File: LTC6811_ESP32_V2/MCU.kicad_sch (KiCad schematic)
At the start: 17 parts, among them J18 B2P-VH-B, J8 JTAG /NC, U8 ESP32-DevKitC V4, U9 LTC6820

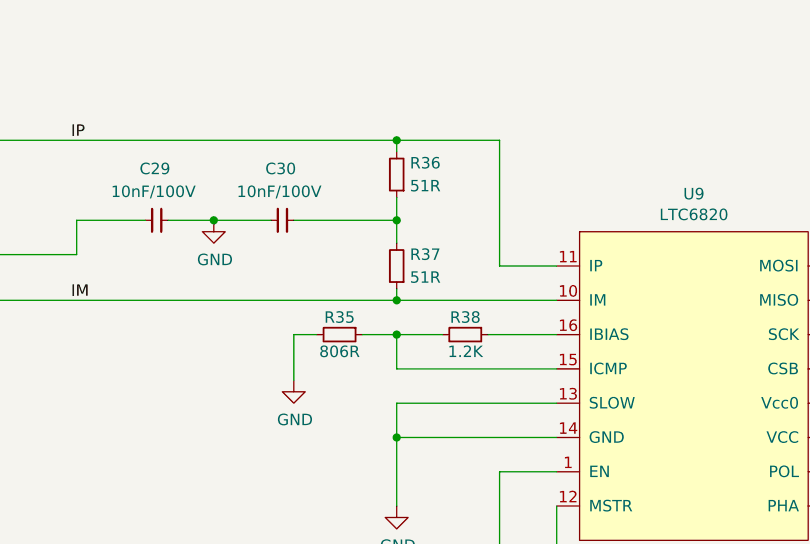
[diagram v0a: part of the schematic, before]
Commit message: Add files via upload
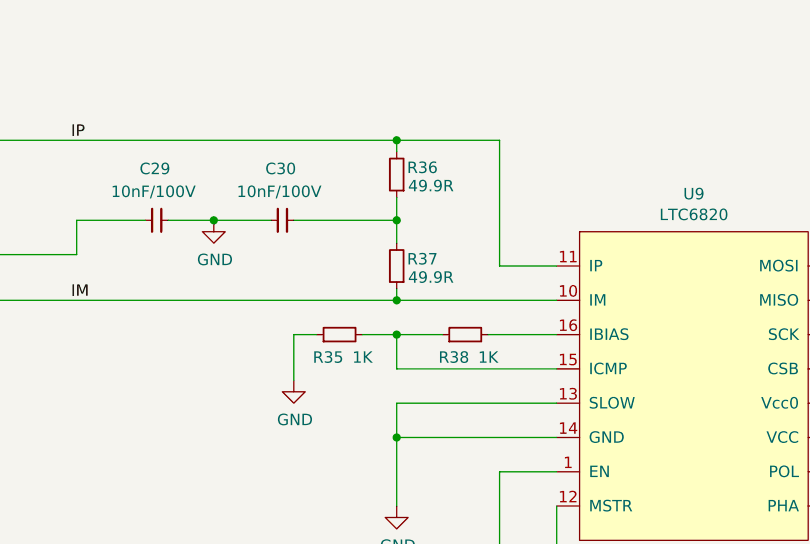
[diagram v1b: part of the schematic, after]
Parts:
- removed R35: 806R, Resistor_SMD:R_0603_1608Metric, symbol Device:R_Small
- removed R36, R37: 51R, Resistor_SMD:R_0603_1608Metric, symbol Device:R_Small
- removed R38: 1.2K, Resistor_SMD:R_0603_1608Metric, symbol Device:R_Small
- added R35, R38: 1K, Resistor_SMD:R_0603_1608Metric, symbol Library:R_Small
- added R36, R37: 49.9R, Resistor_SMD:R_0402_1005Metric, symbol Library:R_Small
- C27, C28, C31, C32: symbol Device:C -> Library:C
- C29, C30: footprint Capacitor_SMD:C_0603_1608Metric -> Capacitor_SMD:C_0402_1005Metric; symbol Device:C -> Library:C; Link https://www.digikey.jp/en/products/detail/murata-electronic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 -> https://www.digikey.jp/en/products/detail/kemet/C0402C103K1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; MPN GCM188R72A103KA37D -> C0402C103K1RACAUTO
- J18: symbol Connector_Generic:Conn_01x02 -> Library:Conn_01x02
- J8: symbol Connector_Generic:Conn_01x04 -> Library:Conn_01x04
- R34: symbol Device:R_Small -> Library:R_Small; Link https://www.digikey.jp/en/products/detail/stackpole-electronics-inc/RMCF0603FT10K0/1761235?s=N4IgTCBcDaIEoFkDCAxADANjQZhQFQEY0BpNEAXQF8g -> https://www.digikey.jp/en/products/detail/stackpole-electronics-inc/RMCF0603JT10K0/1758104; MPN RMCF0603FT10K0 -> RMCF0603JT10K0
- R39: symbol Device:R_Small -> Library:R_Small
- TR2: symbol ENNOID:HM2108NL -> Library:HM2108NL
- U8: symbol MCU_Module:ESP32-DevKitC V4 -> Library:ESP32-DevKitC V4_4
- U9: symbol ENNOID:LTC6820 -> Library:LTC6820
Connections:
- net GND: now also R35.1
- net IM: now also R37.1
- net IP: now also R36.2
- net at C30.2: now also R36.1, R37.2
- net at U9.16 (IBIAS): now also R38.2
- net at U9.15 (ICMP): now also R35.2, R38.1

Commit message: Add files via upload
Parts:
- C29, C30: footprint Capacitor_SMD:C_0402_1005Metric -> Capacitor_SMD:C_0603_1608Metric; Link https://www.digikey.jp/en/products/detail/kemet/C0402C103K1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 -> https://www.digikey.jp/en/products/detail/kemet/C0603X103K1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; MPN C0402C103K1RACAUTO -> C0603X103K1RAC3316
- R36, R37: footprint Resistor_SMD:R_0402_1005Metric -> Resistor_SMD:R_0603_1608Metric; Link https://www.digikey.jp/en/products/detail/yageo/RC0402FR-07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 -> https://www.digikey.jp/en/products/detail/panasonic-electro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; MPN RC0402FR-0749R9L -> ERJ-3EKF49R9V
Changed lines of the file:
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@@
 			)
 		)
-		(property "Footprint" "Capacitor_SMD:C_0402_1005Metric"
+		(property "Footprint" "Capacitor_SMD:C_0603_1608Metric"
 			(at 123.19 70.1548 0)
 			(effects
@@
 			)
 		)
-		(property "Datasheet" "https://content.kemet.com/datasheets/KEM_C1023_X7R_AUTO_SMD.pdf"
+		(property "Datasheet" "https://content.kemet.com/datasheets/KEM_X7R_FT_VW_AUDI.pdf"
 			(at 119.38 71.12 0)
 			(effects
@@
 			)
 		)
-		(property "Description" "10000 pF ±10% 100V Ceramic Capacitor X7R 0402 (1005 Metric)"
+		(property "Description" "10000 pF ±10% 100V Ceramic Capacitor X7R 0603 (1608 Metric)"
 			(at 119.38 71.12 0)
 			(effects
@@
 			)
 		)
-		(property "MPN" "C0402C103K1RACAUTO"
+		(property "MPN" "C0603X103K1RAC3316"
 			(at 119.38 71.12 0)
 			(effects
@@
 			)
 		)
-		(property "Link" "https://www.digikey.jp/en/products/detail/kemet/C0402C103K1RACAUTO/19200876"
+		(property "Link" "https://www.digikey.jp/en/products/detail/kemet/C0603X103K1RAC3316/10315782"
 			(at 119.38 71.12 0)
 			(effects
@@
 			)
 		)
-		(property "Footprint" "Capacitor_SMD:C_0402_1005Metric"
+		(property "Footprint" "Capacitor_SMD:C_0603_1608Metric"
 			(at 109.22 70.1548 0)
 			(effects
@@
 			)
 		)
-		(property "Datasheet" "https://content.kemet.com/datasheets/KEM_C1023_X7R_AUTO_SMD.pdf"
+		(property "Datasheet" "https://content.kemet.com/datasheets/KEM_X7R_FT_VW_AUDI.pdf"
 			(at 105.41 71.12 0)
 			(effects
@@
 			)
 		)
-		(property "Description" "10000 pF ±10% 100V Ceramic Capacitor X7R 0402 (1005 Metric)"
+		(property "Description" "10000 pF ±10% 100V Ceramic Capacitor X7R 0603 (1608 Metric)"
 			(at 105.41 71.12 0)
 			(effects
@@
 			)
 		)
-		(property "MPN" "C0402C103K1RACAUTO"
+		(property "MPN" "C0603X103K1RAC3316"
 			(at 105.41 71.12 0)
 			(effects
@@
 			)
 		)
-		(property "Link" "https://www.digikey.jp/en/products/detail/kemet/C0402C103K1RACAUTO/19200876"
+		(property "Link" "https://www.digikey.jp/en/products/detail/kemet/C0603X103K1RAC3316/10315782"
 			(at 105.41 71.12 0)
 			(effects
@@
 			)
 		)
-		(property "Footprint" "Resistor_SMD:R_0402_1005Metric"
+		(property "Footprint" "Resistor_SMD:R_0603_1608Metric"
 			(at 132.08 76.2 0)
 			(effects
@@
 			)
 		)
-		(property "Datasheet" "https://www.yageo.com/upload/media/product/products/datasheet/rchip/PYu-RC_Group_51_RoHS_L_12.pdf"
+		(property "Datasheet" "https://industrial.panasonic.com/cdbs/www-data/pdf/RDA0000/AOA0000C304.pdf"
 			(at 132.08 76.2 0)
 			(effects
@@
 			)
 		)
-		(property "Description" "49.9 Ohms ±1% 0.063W, 1/16W Chip Resistor 0402 (1005 Metric) Moisture Resistant Thick Film"
+		(property "Description" "49.9 Ohms ±1% 0.1W, 1/10W Chip Resistor 0603 (1608 Metric) Automotive AEC-Q200 Thick Film"
 			(at 132.08 76.2 0)
 			(effects
@@
 			)
 		)
-		(property "Link" "https://www.digikey.jp/en/products/detail/yageo/RC0402FR-0749R9L/726621"
+		(property "Link" "https://www.digikey.jp/en/products/detail/panasonic-electronic-components/ERJ-3EKF49R9V/196378"
 			(at 132.08 76.2 0)
 			(effects
@@
 			)
 		)
-		(property "MPN" "RC0402FR-0749R9L"
+		(property "MPN" "ERJ-3EKF49R9V"
 			(at 132.08 76.2 0)
 			(effects
@@
 			)
 		)
-		(property "Footprint" "Resistor_SMD:R_0402_1005Metric"
+		(property "Footprint" "Resistor_SMD:R_0603_1608Metric"
 			(at 132.08 66.04 0)
 			(effects
@@
 			)
 		)
-		(property "Datasheet" "https://www.yageo.com/upload/media/product/products/datasheet/rchip/PYu-RC_Group_51_RoHS_L_12.pdf"
+		(property "Datasheet" "https://industrial.panasonic.com/cdbs/www-data/pdf/RDA0000/AOA0000C304.pdf"
 			(at 132.08 66.04 0)
 			(effects
@@
 			)
 		)
-		(property "Description" "49.9 Ohms ±1% 0.063W, 1/16W Chip Resistor 0402 (1005 Metric) Moisture Resistant Thick Film"
+		(property "Description" "49.9 Ohms ±1% 0.1W, 1/10W Chip Resistor 0603 (1608 Metric) Automotive AEC-Q200 Thick Film"
 			(at 132.08 66.04 0)
 			(effects
@@
 			)
 		)
-		(property "Link" "https://www.digikey.jp/en/products/detail/yageo/RC0402FR-0749R9L/726621"
+		(property "Link" "https://www.digikey.jp/en/products/detail/panasonic-electronic-components/ERJ-3EKF49R9V/196378"
 			(at 132.08 66.04 0)
 			(effects
@@
 			)
 		)
-		(property "MPN" "RC0402FR-0749R9L"
+		(property "MPN" "ERJ-3EKF49R9V"
 			(at 132.08 66.04 0)
 			(effects
